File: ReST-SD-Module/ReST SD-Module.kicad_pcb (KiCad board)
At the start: 2 copper layers, 18.7 x 28.7 mm, 25 parts

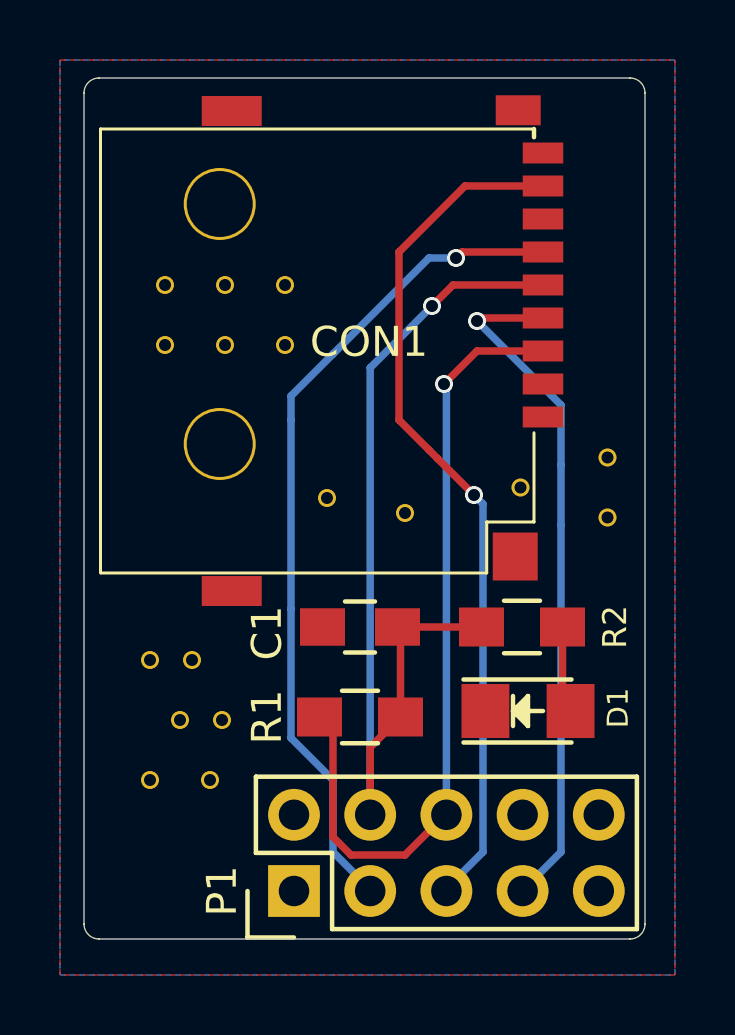
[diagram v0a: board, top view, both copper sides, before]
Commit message: Final release
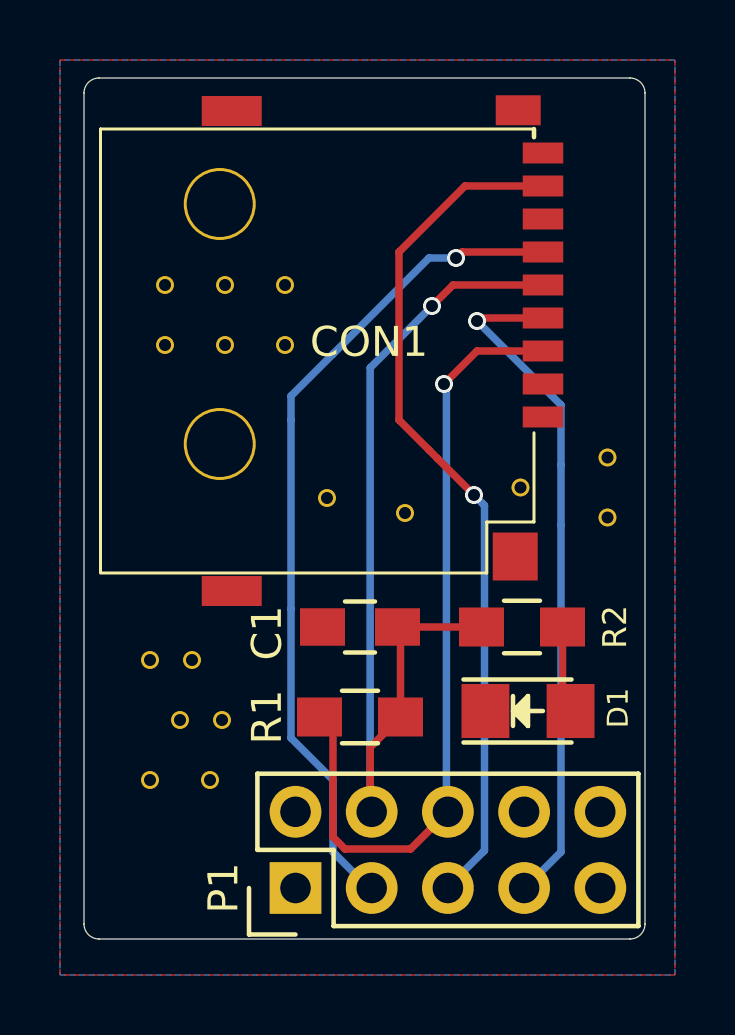
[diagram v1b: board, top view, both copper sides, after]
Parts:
- moved P1 0.11 mm to (141.8, 108.1)
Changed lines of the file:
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@@
     (links 34)
     (no_connects 0)
-    (area 134.794999 81.094999 153.505001 109.805001)
+    (area 134 80.5 154.500001 111.000001)
     (thickness 1.6)
     (drawings 9)
-    (tracks 57)
+    (tracks 59)
     (zones 0)
     (modules 25)
@@
     (visible_elements 7FFFFFFF)
     (pcbplotparams
-      (layerselection 0x00030_80000001)
-      (usegerberextensions false)
+      (layerselection 0x010f0_80000001)
+      (usegerberextensions true)
       (excludeedgelayer true)
       (linewidth 0.100000)
@@
       (psa4output false)
       (plotreference true)
-      (plotvalue true)
+      (plotvalue false)
       (plotinvisibletext false)
       (padsonsilk false)
@@
       (outputformat 1)
       (mirror false)
-      (drillshape 1)
+      (drillshape 0)
       (scaleselection 1)
-      (outputdirectory ""))
+      (outputdirectory "../Gerber/SD Adapter/"))
   )
   (net 0 "")
@@
   )
   (module Pin_Headers:Pin_Header_Straight_2x05 (layer F.Cu)
-    (at 141.8 108.2 90)
+    (at 141.85 108.1 90)
     (descr "Through hole pin header")
     (tags "pin header")
@@
   (segment (start 144.34 105.66) (end 144.34 103.41) (width 0.25) (layer F.Cu) (net 1))
   (segment (start 144.34 103.41) (end 145.35 102.4) (width 0.25) (layer F.Cu) (net 1))
+  (segment (start 146.93 105.56) (end 145.69 106.8) (width 0.25) (layer F.Cu) (net 3))
+  (segment (start 145.69 106.8) (end 143.5 106.8) (width 0.25) (layer F.Cu) (net 3))
+  (segment (start 143.5 106.8) (end 143.1 106.4) (width 0.25) (layer F.Cu) (net 3))
   (segment (start 146.88 105.66) (end 146.88 91.38) (width 0.25) (layer B.Cu) (net 3))
   (segment (start 147.9 90.2) (end 150.1 90.2) (width 0.25) (layer F.Cu) (net 3))
@@
   (segment (start 146.88 91.38) (end 146.8 91.3) (width 0.25) (layer B.Cu) (net 3))
   (segment (start 146.88 105.66) (end 146.84 105.66) (width 0.25) (layer F.Cu) (net 3))
-  (segment (start 146.84 105.66) (end 145.5 107) (width 0.25) (layer F.Cu) (net 3))
-  (segment (start 145.5 107) (end 143.7 107) (width 0.25) (layer F.Cu) (net 3))
-  (segment (start 143.7 107) (end 143.1 106.4) (width 0.25) (layer F.Cu) (net 3))
   (segment (start 143.1 106.4) (end 143.1 102.85) (width 0.25) (layer F.Cu) (net 3))
   (segment (start 143.1 102.85) (end 142.65 102.4) (width 0.25) (layer F.Cu) (net 3))
@@
   (segment (start 143.1 90.3) (end 146.3 87.1) (width 0.25) (layer B.Cu) (net 5))
   (segment (start 144.34 108.2) (end 144.34 107.96) (width 0.25) (layer B.Cu) (net 5))
+  (segment (start 148.1 95.3) (end 148.15 95.35) (width 0.25) (layer B.Cu) (net 6))
+  (segment (start 148.15 95.35) (end 148.15 106.85) (width 0.25) (layer B.Cu) (net 6))
+  (segment (start 148.15 106.85) (end 148.1 106.9) (width 0.25) (layer B.Cu) (net 6))
   (segment (start 146.88 108.2) (end 146.88 108.12) (width 0.25) (layer B.Cu) (net 6))
   (segment (start 146.88 108.12) (end 148.1 106.9) (width 0.25) (layer B.Cu) (net 6))
-  (segment (start 148.1 106.9) (end 148.1 95.3) (width 0.25) (layer B.Cu) (net 6))
   (segment (start 148.1 95.3) (end 147.8 95) (width 0.25) (layer B.Cu) (net 6))
   (via (at 147.8 95) (size 0.6) (drill 0.4) (layers F.Cu B.Cu) (net 6))
